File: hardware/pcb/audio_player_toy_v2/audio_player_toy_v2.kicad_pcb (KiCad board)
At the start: 2 copper layers, 75 x 60 mm, 19 parts, among them J1 Conn_02x05_Odd_Even, U1 ISD2360YYI, U2 BH-AAA-B5AA005

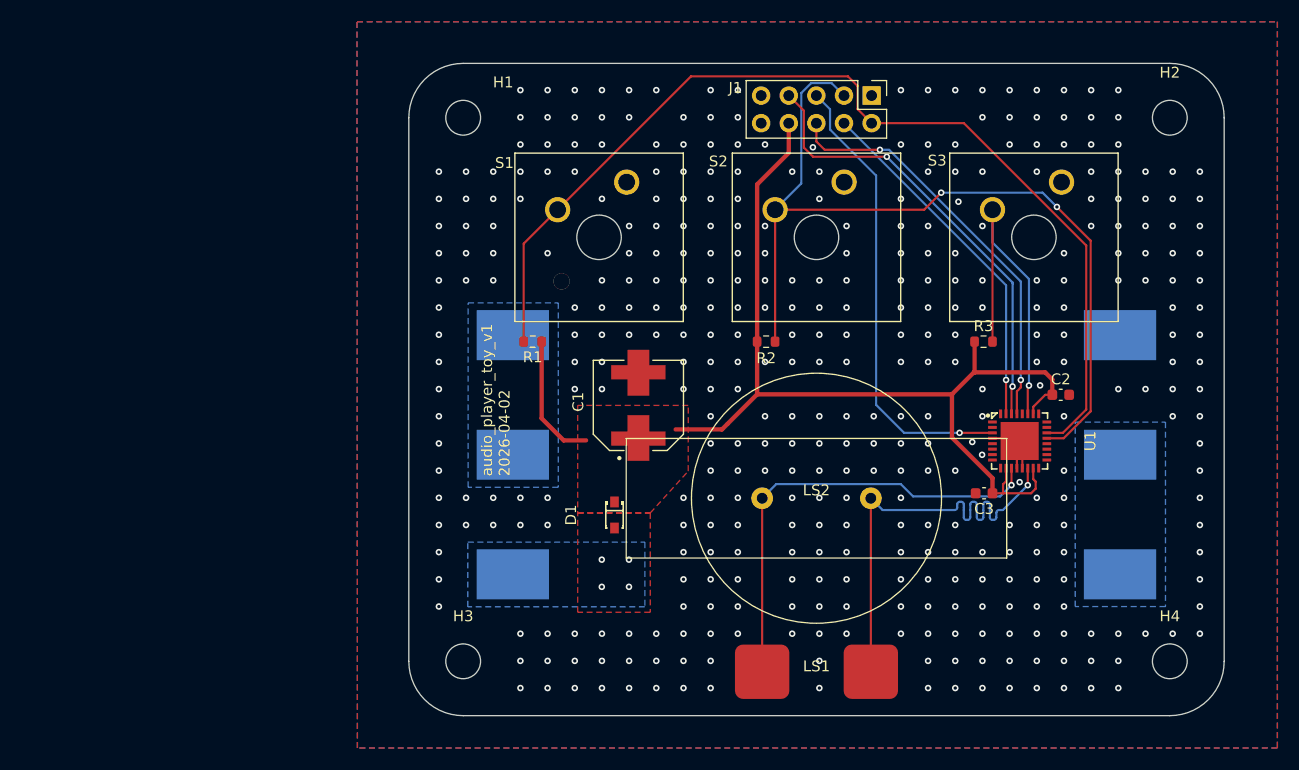
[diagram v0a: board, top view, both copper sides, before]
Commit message: chore: complete finding all footprints, ready to routing, both version
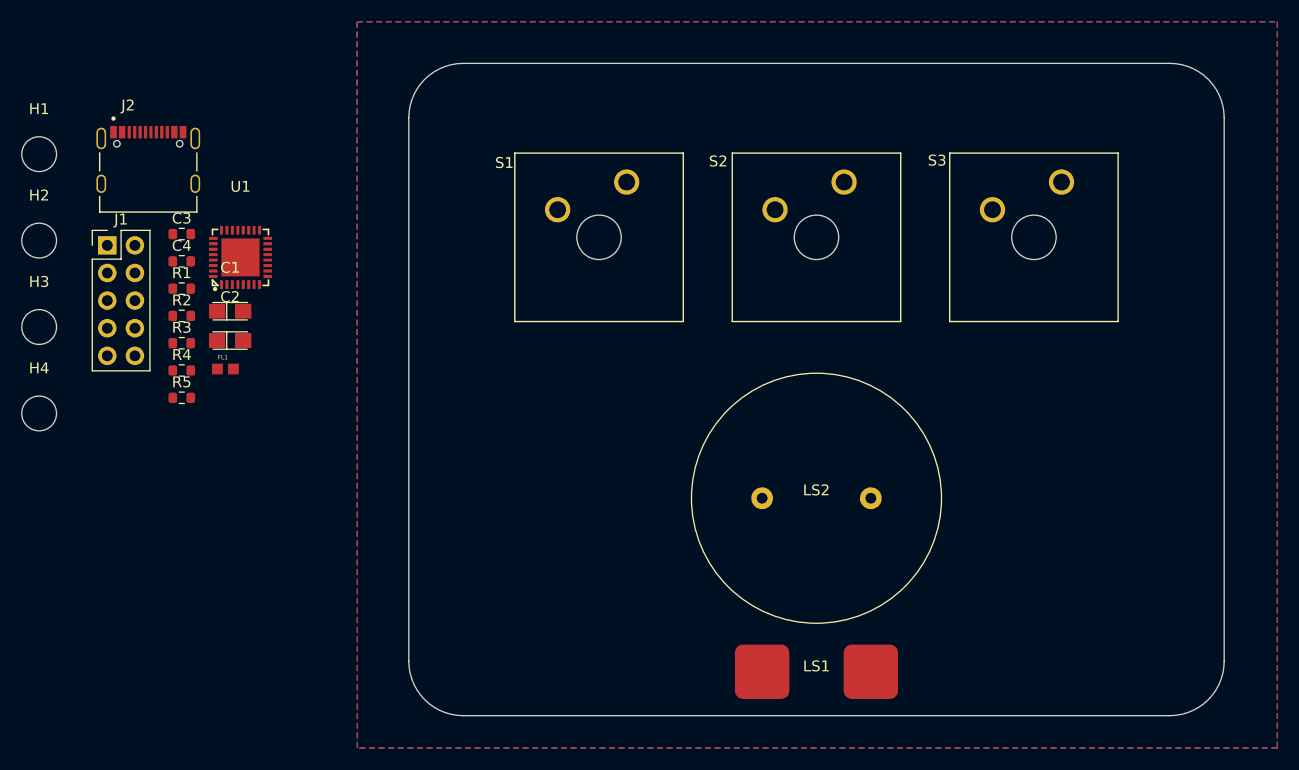
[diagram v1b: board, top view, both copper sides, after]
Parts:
- removed D1: 1N5817WS_C727114, .pretty:SOD-323_L1.8-W1.3-LS2.5-FD
- removed U2: BH-AAA-B5AA005, .pretty:BAT-SMD_BH-AAA-B5AA005
- added C4: 10uF, Resistor_SMD:R_0603_1608Metric, F.Cu at (79.1, 118.2)
- added FL1: BLM18PG601SN1, .pretty:BEADC1608X95N, F.Cu at (83.1, 128.1)
- added J2: TYPE-C-31-M-12, .pretty:HRO_TYPE-C-31-M-12, F.Cu at (76.0, 111.1)
- added R4: 10K, Resistor_SMD:R_0603_1608Metric, F.Cu at (79.1, 128.2)
- added R5: 5.1K, Resistor_SMD:R_0603_1608Metric, F.Cu at (79.1, 130.8)
- C1: value EEEFK1A221V -> 47uF; footprint .pretty:CAP_EEEFK1A221V -> .pretty:CASE-A_3216
- C2: value 4.7uF -> 47uF; footprint Capacitor_SMD:C_0603_1608Metric -> .pretty:CASE-A_3216
- C3: value 4.7uF -> 0.1uF; footprint Capacitor_SMD:C_0603_1608Metric -> Resistor_SMD:R_0603_1608Metric
- R1: value 10K -> 5.1K
- moved H4 106.5 mm to (66.0, 132.2)
- moved H2 104.6 mm to (66.0, 116.3)
- moved C3 77.6 mm to (79.1, 115.7), turned to 0 degrees
- moved C2 76.6 mm to (83.6, 125.5)
- moved R3 73.8 mm to (79.1, 125.7)
- moved U1 73.6 mm to (84.5, 117.8), turned to 0 degrees
- moved J1 71.6 mm to (72.3, 116.7), turned to 0 degrees
- moved R2 53.8 mm to (79.1, 123.2)
- moved H3 49.7 mm to (66.0, 124.2)
- moved H1 39.1 mm to (66.0, 108.3)
- moved C1 38.5 mm to (83.6, 122.8), turned to 0 degrees
- moved R1 32.6 mm to (79.1, 120.7), turned to 0 degrees
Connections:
- C1 pad 1: BAT+ -> VCCD
- C2 pad 1: BAT+ -> VCCD
- C3 pad 1: BAT+ -> VCCD
- J1 pad 8: BAT+ -> VCCD
- R1 pad 1: BAT+ -> Net-(J2-CC1)
- R1 pad 2: RDY/BSYB -> GND
- R2 pad 1: BAT+ -> VCCD
- R2 pad 2: INTB -> RDY/BSYB
- R3 pad 1: BAT+ -> VCCD
- R3 pad 2: GPIO5 -> INTB
- U1 pad 10: BAT+ -> VCCD
- U1 pad 15: BAT+ -> VCCD
- U1 pad 26: BAT+ -> VCCD
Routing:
- net BAT+: track 101.5 -> 0.00 mm
- net RDY/BSYB: track 94.4 -> 0.00 mm
- net INTB: track 80.9 -> 0.00 mm, vias 2 -> 0
- net MOSI: track 42.5 -> 0.00 mm, vias 1 -> 0
- net SPK+: track 41.9 -> 0.00 mm, vias 1 -> 0
- net SCLK: track 41.8 -> 0.00 mm, vias 2 -> 0
- net SPK-: track 41.8 -> 0.00 mm, vias 1 -> 0
- net MISO: track 38.1 -> 0.00 mm, vias 2 -> 0
- net SSB: track 32.9 -> 0.00 mm, vias 1 -> 0
- net GPIO5: track 32.3 -> 0.00 mm, vias 1 -> 0
- net GND: track 7.81 -> 0.00 mm, vias 390 -> 0
- net Net-(D1-A): vias 4 -> 0
- removed copper zone on F.Cu, net BAT+
- removed copper zone on B.Cu, net Net-(D1-A)
- removed copper zone on F.Cu, net Net-(D1-A)
- removed copper zone on B.Cu, net Net-(U2-+-Pad2)
- removed copper zone on B.Cu, net Net-(U2-+-Pad6)
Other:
- board text removed: "audio_player_toy_v1 2026-04-02"
